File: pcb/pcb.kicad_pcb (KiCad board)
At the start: 2 copper layers, 104.6 x 75.2 mm, 10 parts

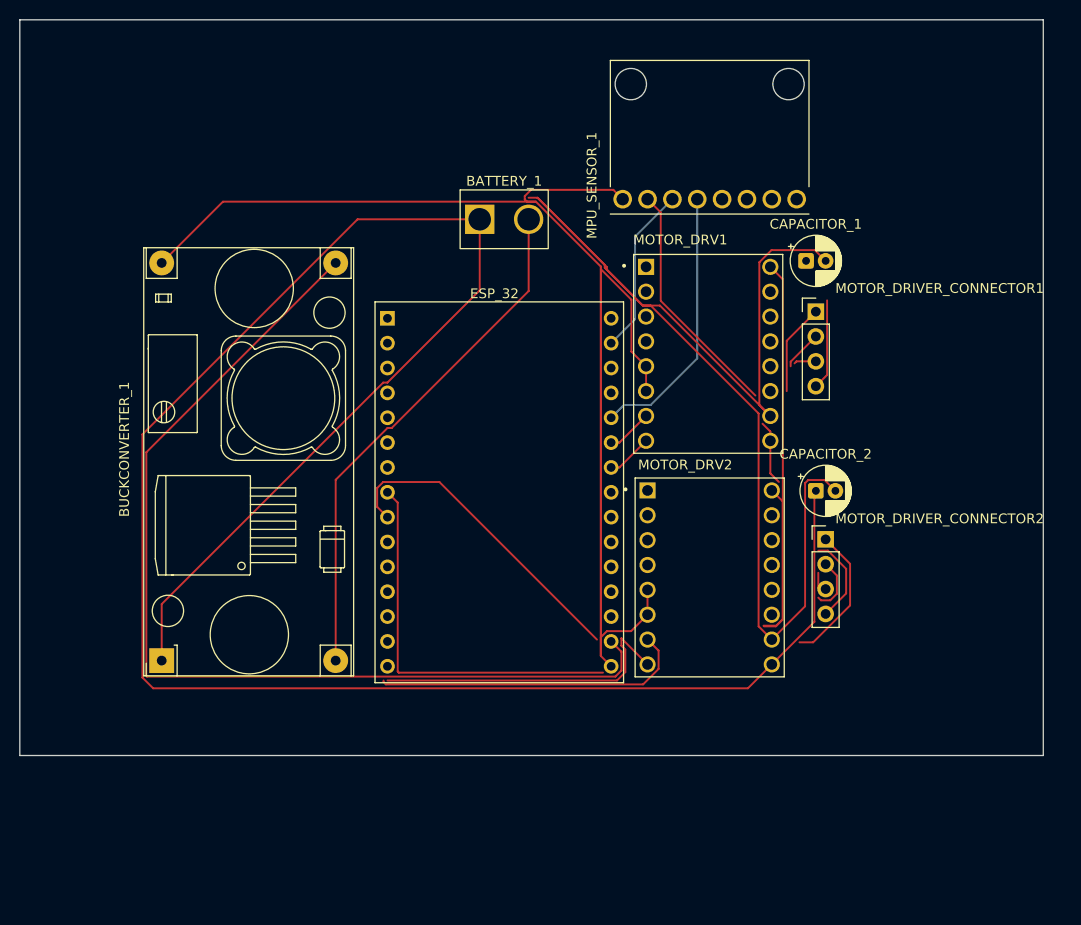
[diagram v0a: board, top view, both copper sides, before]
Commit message: Finalized PCB version 1
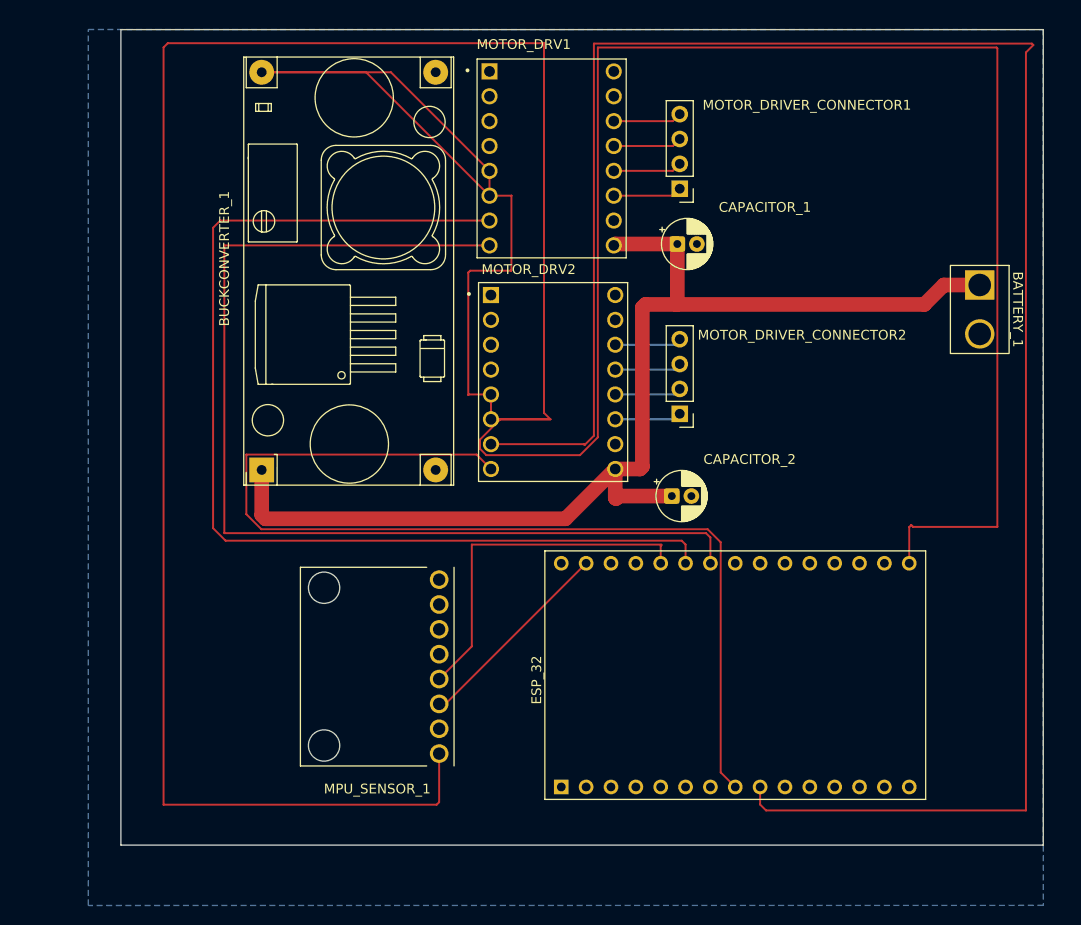
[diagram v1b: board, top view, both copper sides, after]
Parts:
- BATTERY_1: footprint SelfBalancingRobot:Untitled -> SelfBalancingRobot:Battery_Connection_01x02
- moved MPU_SENSOR_1 63.9 mm to (98.0, 147.6), turned to 180 degrees
- moved ESP_32 51.1 mm to (116.8, 159.9), turned to 90 degrees
- moved BATTERY_1 50.1 mm to (156.6, 106.6), turned to -90 degrees
- moved MOTOR_DRV2 25.6 mm to (116.0, 118.5)
- moved MOTOR_DRV1 25.6 mm to (115.8, 95.7)
- moved BUCKCONVERTER_1 22.0 mm to (86.2, 127.5)
- moved MOTOR_DRIVER_CONNECTOR2 19.7 mm to (128.9, 121.8), turned to 180 degrees
- moved MOTOR_DRIVER_CONNECTOR1 18.7 mm to (128.9, 98.8), turned to 180 degrees
- moved CAPACITOR_2 14.7 mm to (128.1, 130.2)
- moved CAPACITOR_1 13.3 mm to (128.7, 104.4)
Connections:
- BATTERY_1 pad 2: Net-(BATTERY_1-Pin_2) -> GND
- BUCKCONVERTER_1 pad 2: Net-(BATTERY_1-Pin_2) -> GND
- BUCKCONVERTER_1 pad 3: Net-(BUCKCONVERTER_1-Pin_3) -> GND
- CAPACITOR_1 pad 2: Net-(BATTERY_1-Pin_2) -> GND
- CAPACITOR_2 pad 2: Net-(BATTERY_1-Pin_2) -> GND
- ESP_32 pad 17: Net-(BUCKCONVERTER_1-Pin_3) -> GND
- MOTOR_DRV1 pad 10: Net-(BATTERY_1-Pin_2) -> GND
- MOTOR_DRV1 pad 16: Net-(BUCKCONVERTER_1-Pin_3) -> GND
- MOTOR_DRV2 pad 10: Net-(BATTERY_1-Pin_2) -> GND
- MOTOR_DRV2 pad 16: Net-(BUCKCONVERTER_1-Pin_3) -> GND
- MPU_SENSOR_1 pad 2: Net-(BUCKCONVERTER_1-Pin_3) -> GND
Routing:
- net Net-(BUCKCONVERTER_1-3v3): track 168.1 -> 449.3 mm
- net Net-(BATTERY_1-Pin_2): track 188.1 -> 0.00 mm
- net Net-(BUCKCONVERTER_1-Pin_3): track 181.7 -> 0.00 mm
- net Net-(ESP_32-Pin_9): track 65.3 -> 203.7 mm
- net Net-(ESP_32-Pin_25): track 4.70 -> 110.1 mm
- net Net-(ESP_32-Pin_24): track 4.70 -> 109.0 mm
- net Net-(BATTERY_1-BAT+): track 219.3 -> 119.3 mm
- net Net-(ESP_32-Pin_8): track 71.8 -> 107.0 mm
- net Net-(ESP_32-Pin_26): track 27.6 -> 36.4 mm
- net Net-(MOTOR_DRIVER_CONNECTOR2-B2): track 14.5 -> 6.82 mm
- net Net-(MOTOR_DRIVER_CONNECTOR1-A1): track 2.26 -> 7.04 mm
- net Net-(MOTOR_DRIVER_CONNECTOR2-A1): track 2.36 -> 6.82 mm
- net Net-(ESP_32-Pin_29): track 17.3 -> 21.0 mm
- net Net-(MOTOR_DRIVER_CONNECTOR1-B1): track 4.11 -> 7.04 mm
- net Net-(MOTOR_DRIVER_CONNECTOR1-B2): track 9.35 -> 7.04 mm
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- added copper zone on B.Cu, net GND
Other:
- board size 104.6 x 75.2 mm -> 94.3 x 83.3 mm
